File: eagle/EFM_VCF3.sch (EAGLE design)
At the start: 44 parts, among them IC1 LM13700N, IC2 TL084P, Q3 2N3906, Q4 2N3906, U1 POWER

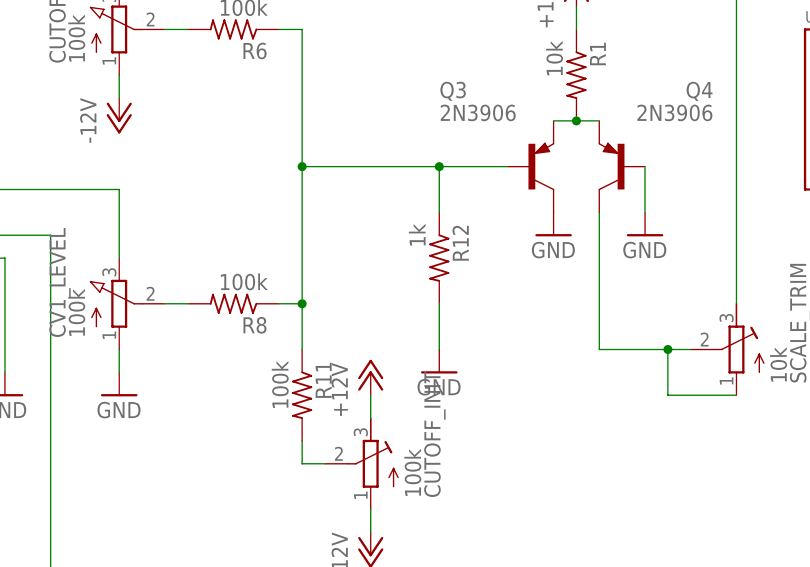
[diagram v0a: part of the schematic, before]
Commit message: gcode
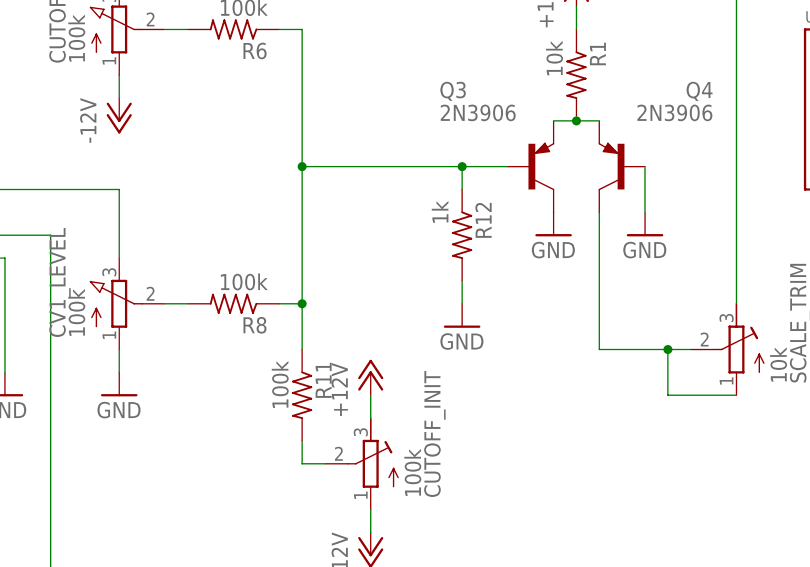
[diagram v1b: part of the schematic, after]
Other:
- moved on the sheet: R12
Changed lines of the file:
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@@
 <?xml version="1.0" encoding="utf-8"?>
 <!DOCTYPE eagle SYSTEM "eagle.dtd">
-<eagle version="7.2.0">
+<eagle version="7.1.0">
 <drawing>
 <settings>
@@
 <instance part="C1" gate="G$1" x="132.08" y="48.26"/>
 <instance part="C2" gate="G$1" x="132.08" y="33.02"/>
-<instance part="R12" gate="G$1" x="-10.16" y="20.32" rot="R270"/>
-<instance part="GND9" gate="1" x="-10.16" y="7.62"/>
+<instance part="R12" gate="G$1" x="-7.62" y="22.86" rot="R270"/>
+<instance part="GND9" gate="1" x="-7.62" y="12.7"/>
 <instance part="Q3" gate="G$1" x="0" y="30.48"/>
 <instance part="Q4" gate="G$1" x="10.16" y="30.48" rot="MR0"/>
@@
 <segment>
 <pinref part="R12" gate="G$1" pin="2"/>
-<wire x1="-10.16" y1="10.16" x2="-10.16" y2="15.24" width="0.1524" layer="91"/>
+<wire x1="-7.62" y1="15.24" x2="-7.62" y2="17.78" width="0.1524" layer="91"/>
 <pinref part="GND9" gate="1" pin="GND"/>
 </segment>
@@
 <wire x1="-25.4" y1="30.48" x2="-25.4" y2="15.24" width="0.1524" layer="91"/>
 <wire x1="-25.4" y1="15.24" x2="-27.94" y2="15.24" width="0.1524" layer="91"/>
-<wire x1="-2.54" y1="30.48" x2="-10.16" y2="30.48" width="0.1524" layer="91"/>
+<wire x1="-2.54" y1="30.48" x2="-7.62" y2="30.48" width="0.1524" layer="91"/>
 <pinref part="R11" gate="G$1" pin="1"/>
-<wire x1="-10.16" y1="30.48" x2="-25.4" y2="30.48" width="0.1524" layer="91"/>
+<wire x1="-7.62" y1="30.48" x2="-25.4" y2="30.48" width="0.1524" layer="91"/>
 <wire x1="-25.4" y1="10.16" x2="-25.4" y2="15.24" width="0.1524" layer="91"/>
 <junction x="-25.4" y="15.24"/>
 <pinref part="R12" gate="G$1" pin="1"/>
-<wire x1="-10.16" y1="25.4" x2="-10.16" y2="30.48" width="0.1524" layer="91"/>
-<junction x="-10.16" y="30.48"/>
+<wire x1="-7.62" y1="27.94" x2="-7.62" y2="30.48" width="0.1524" layer="91"/>
+<junction x="-7.62" y="30.48"/>
 <pinref part="Q3" gate="G$1" pin="B"/>
 <junction x="-25.4" y="30.48"/>
